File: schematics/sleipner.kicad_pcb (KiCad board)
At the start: 2 copper layers, 171.4 x 129.5 mm, 129 parts, among them J1 Conn_01x04_Male, J10 AudioJack3, J11 AudioJack3, J12 AudioJack3, J13 AudioJack3, J2 Barrel_Jack_Switch, J3 AudioJack3, J4 AudioJack3, J5 AudioJack3, J6 AudioJack3, J7 AudioJack3, J8 AudioJack3, J9 AudioJack3, Q1 BC337, Q2 BC337, Q3 BC337, Q4 BC337, Q5 BC337, Q6 BC337, Q7 BC337, Q8 BC337, Q9 BC337, SW1 SW_DIP_x01, SW10 SW_DIP_x01, SW11 Rotary_Encoder, SW12 SW_DIP_x01, SW13 SW_DIP_x01, SW14 SW_DIP_x01, SW15 SW_DIP_x01, SW16 SW_DIP_x01, SW17 SW_DIP_x01, SW18 SW_DIP_x01, SW19 SW_DIP_x01, SW2 SW_DIP_x01, SW3 SW_DIP_x01, SW4 SW_DIP_x01, SW5 SW_DIP_x01, SW6 SW_DIP_x01, SW7 SW_DIP_x01, SW8 SW_DIP_x01, SW9 SW_DIP_x01, U1 L7805, U2 ATmega32-16PU, U3 L7812, U4 74LS259, U5 MCP4922-EP, U6 TLC274, Y1 16 MHz

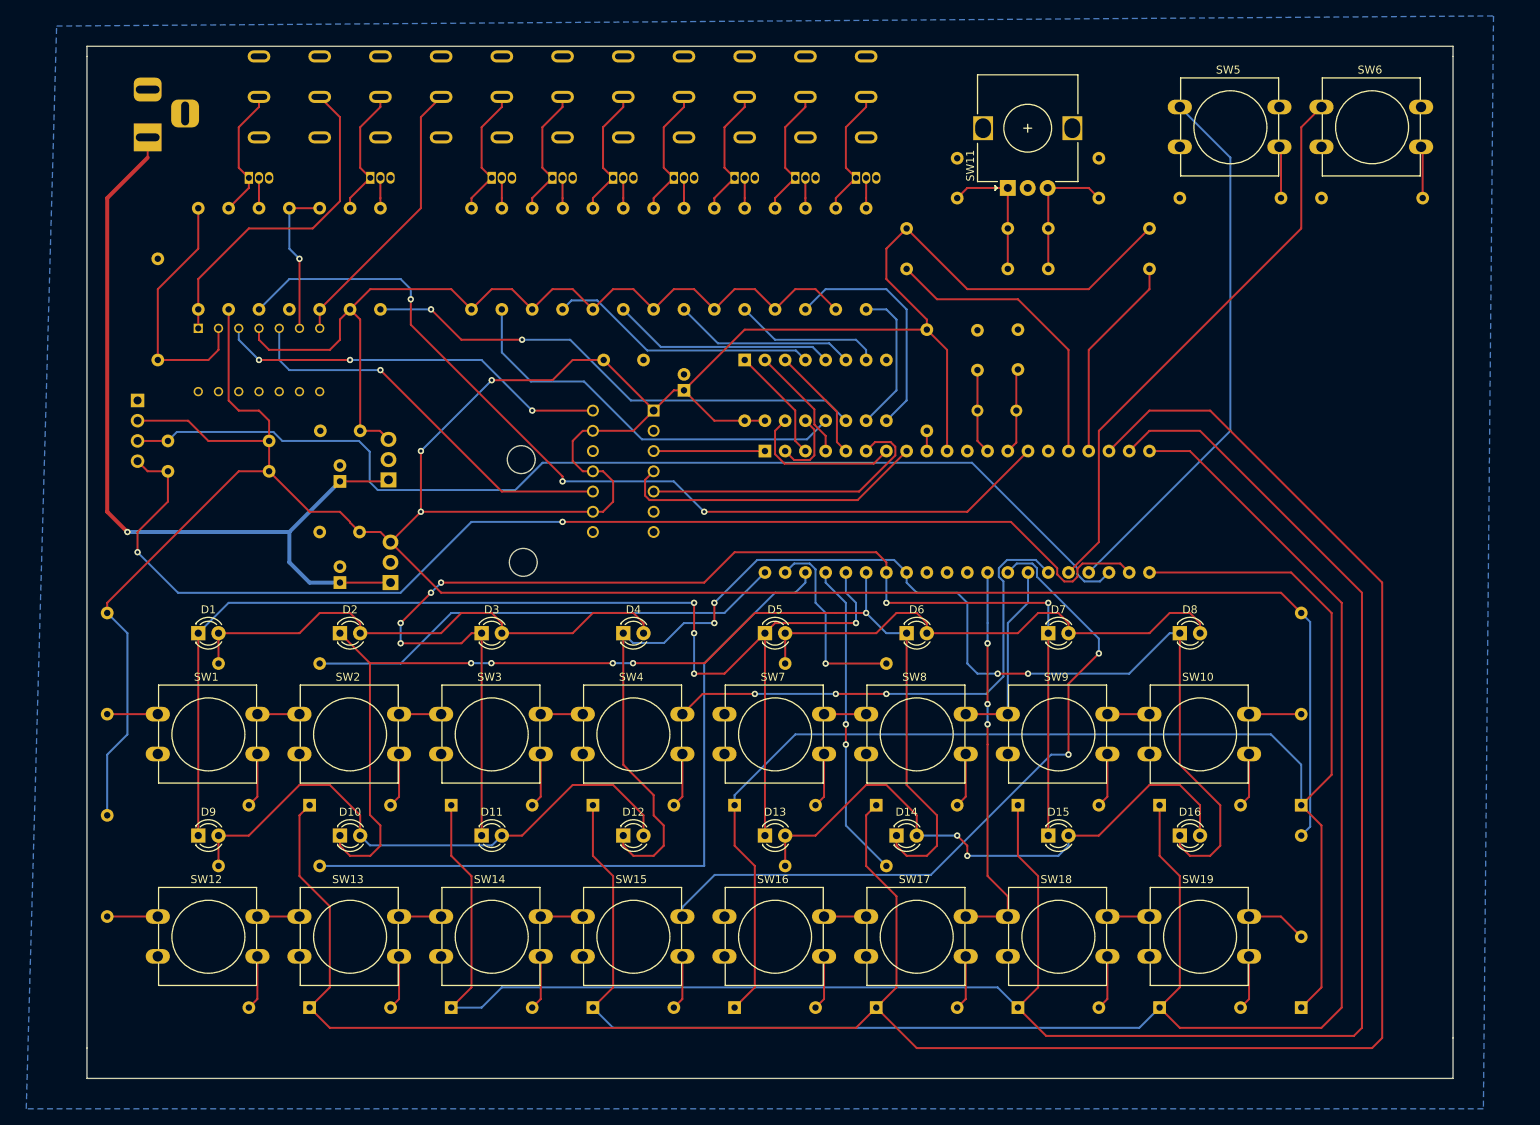
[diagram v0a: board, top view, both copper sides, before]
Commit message: Redo the PCB
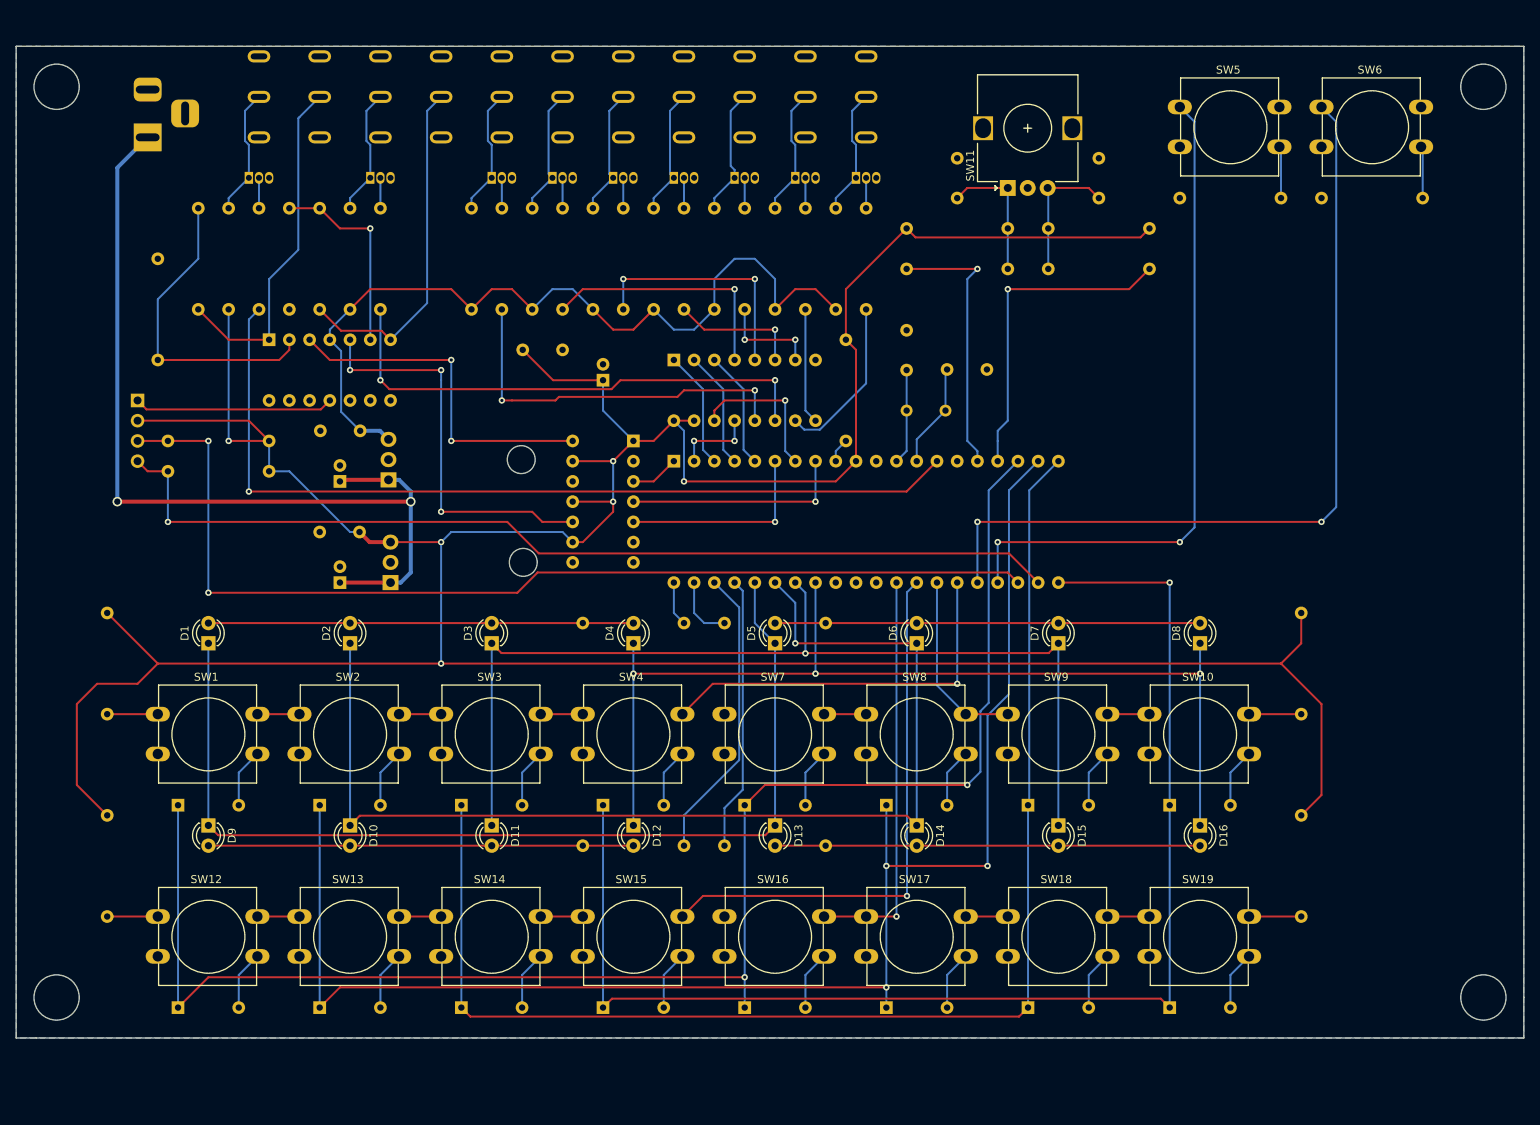
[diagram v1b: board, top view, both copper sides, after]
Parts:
- U5: value MCP4922-EP -> MCP4922; footprint mcp4922:DIP254P762X533-14 -> Package_DIP:DIP-14_W7.62mm
- U6: footprint tlc274:DIP794W45P254L1969H508Q14 -> Package_DIP:DIP-14_W7.62mm
- moved R1 46.0 mm to (134.6, 109.2)
- moved R3 45.8 mm to (134.6, 137.2)
- moved D17 16.5 mm to (83.8, 132.1), turned to 0 degrees
- moved D18 16.5 mm to (101.6, 132.1), turned to 0 degrees
- moved D25 16.5 mm to (83.8, 157.5), turned to 0 degrees
- moved D26 16.5 mm to (101.6, 157.5), turned to 0 degrees
- moved D19 16.5 mm to (119.4, 132.1), turned to 0 degrees
- moved D20 16.5 mm to (137.2, 132.1), turned to 0 degrees
- moved D21 16.5 mm to (154.9, 132.1), turned to 0 degrees
- moved D22 16.5 mm to (172.7, 132.1), turned to 0 degrees
- moved D23 16.5 mm to (190.5, 132.1), turned to 0 degrees
- moved D24 16.5 mm to (208.3, 132.1), turned to 0 degrees
- moved D27 16.5 mm to (119.4, 157.5), turned to 0 degrees
- moved D28 16.5 mm to (137.2, 157.5), turned to 0 degrees
- moved D29 16.5 mm to (154.9, 157.5), turned to 0 degrees
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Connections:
- J10 pad R: Net-(J10-PadR) -> (no net)
- J11 pad R: Net-(J11-PadR) -> (no net)
- J12 pad R: Net-(J12-PadR) -> (no net)
- J13 pad R: Net-(J13-PadR) -> (no net)
- J2 pad 3: Net-(J2-Pad3) -> (no net)
- J3 pad R: Net-(J3-PadR) -> (no net)
- J4 pad R: Net-(J4-PadR) -> (no net)
- J5 pad R: Net-(J5-PadR) -> (no net)
- J6 pad R: Net-(J6-PadR) -> (no net)
- J7 pad R: Net-(J7-PadR) -> (no net)
- J8 pad R: Net-(J8-PadR) -> (no net)
- J9 pad R: Net-(J9-PadR) -> (no net)
- U2 pad 15: Net-(U2-Pad15) -> (no net)
- U2 pad 30: Net-(U2-Pad30) -> (no net)
- U2 pad 32: Net-(U2-Pad32) -> (no net)
- U5 pad 2: Net-(U5-Pad2) -> (no net)
- U5 pad 6: Net-(U5-Pad6) -> (no net)
- U5 pad 7: Net-(U5-Pad7) -> (no net)
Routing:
- net BtnRow1: track 299.0 -> 195.8 mm, vias 0 -> 2
- net BtnRow2: track 266.6 -> 189.1 mm, vias 0 -> 3
- net BtnRow3: track 236.0 -> 167.6 mm
- net LedCol1: track 60.6 -> 5.61 mm
- net LedCol3: track 91.8 -> 37.2 mm
- net LedRow4: track 161.7 -> 128.3 mm, vias 4 -> 3
- net Net-(SW6-Pad1): track 71.6 -> 104.4 mm, vias 0 -> 2
- net LedRow3: track 158.4 -> 127.3 mm, vias 6 -> 1
- net Net-(J1-Pad4): track 151.9 -> 123.1 mm, vias 2 -> 1
- net LedRow1: track 153.3 -> 126.5 mm, vias 4 -> 0
- net GND: track 0.00 -> 25.1 mm
- net BtnRow4: track 187.9 -> 164.8 mm, vias 0 -> 1
- net BtnCol3: track 112.3 -> 91.3 mm, vias 2 -> 1
- net Net-(D13-Pad2): track 73.7 -> 53.3 mm, vias 2 -> 0
- net +5V: track 479.6 -> 459.8 mm, vias 3 -> 6
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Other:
- board size 171.4 x 129.5 mm -> 189.2 x 124.5 mm
